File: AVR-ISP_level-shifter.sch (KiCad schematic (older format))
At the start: 24 parts, among them Q1 BSS138, Q2 BSS138, Q3 BSS138, Q4 BSS138, Q5 BSS138, Q6 BSS138, Q7 BSS138, Q8 BSS138, SW1 APEM 25439NH, U1 AMS1117-3.3

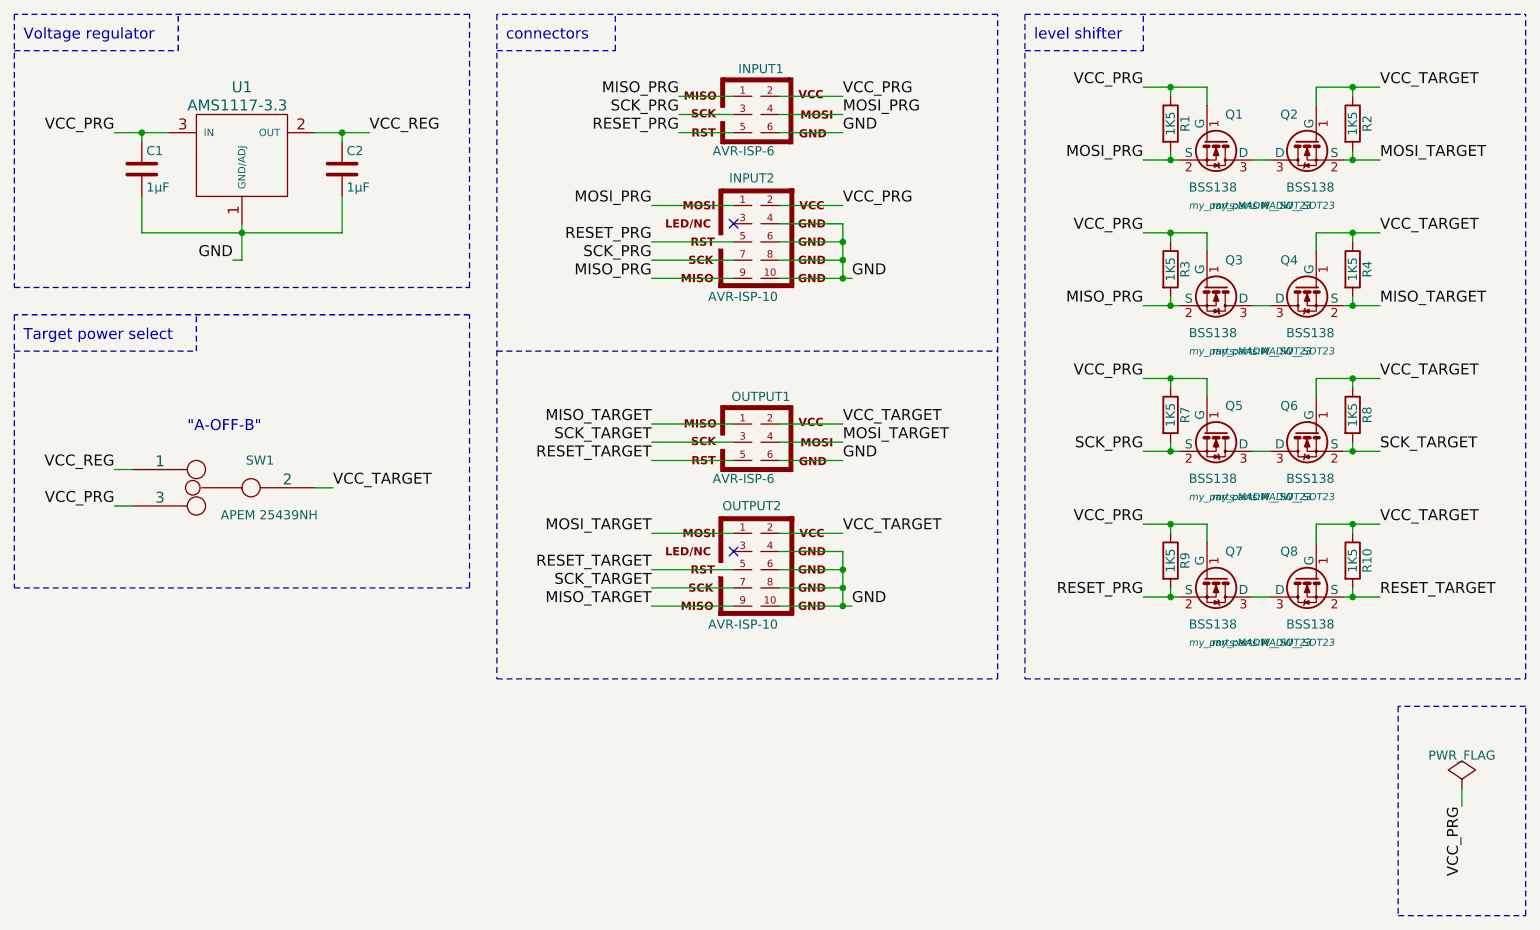
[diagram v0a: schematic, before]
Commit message: Changed a few footprints.
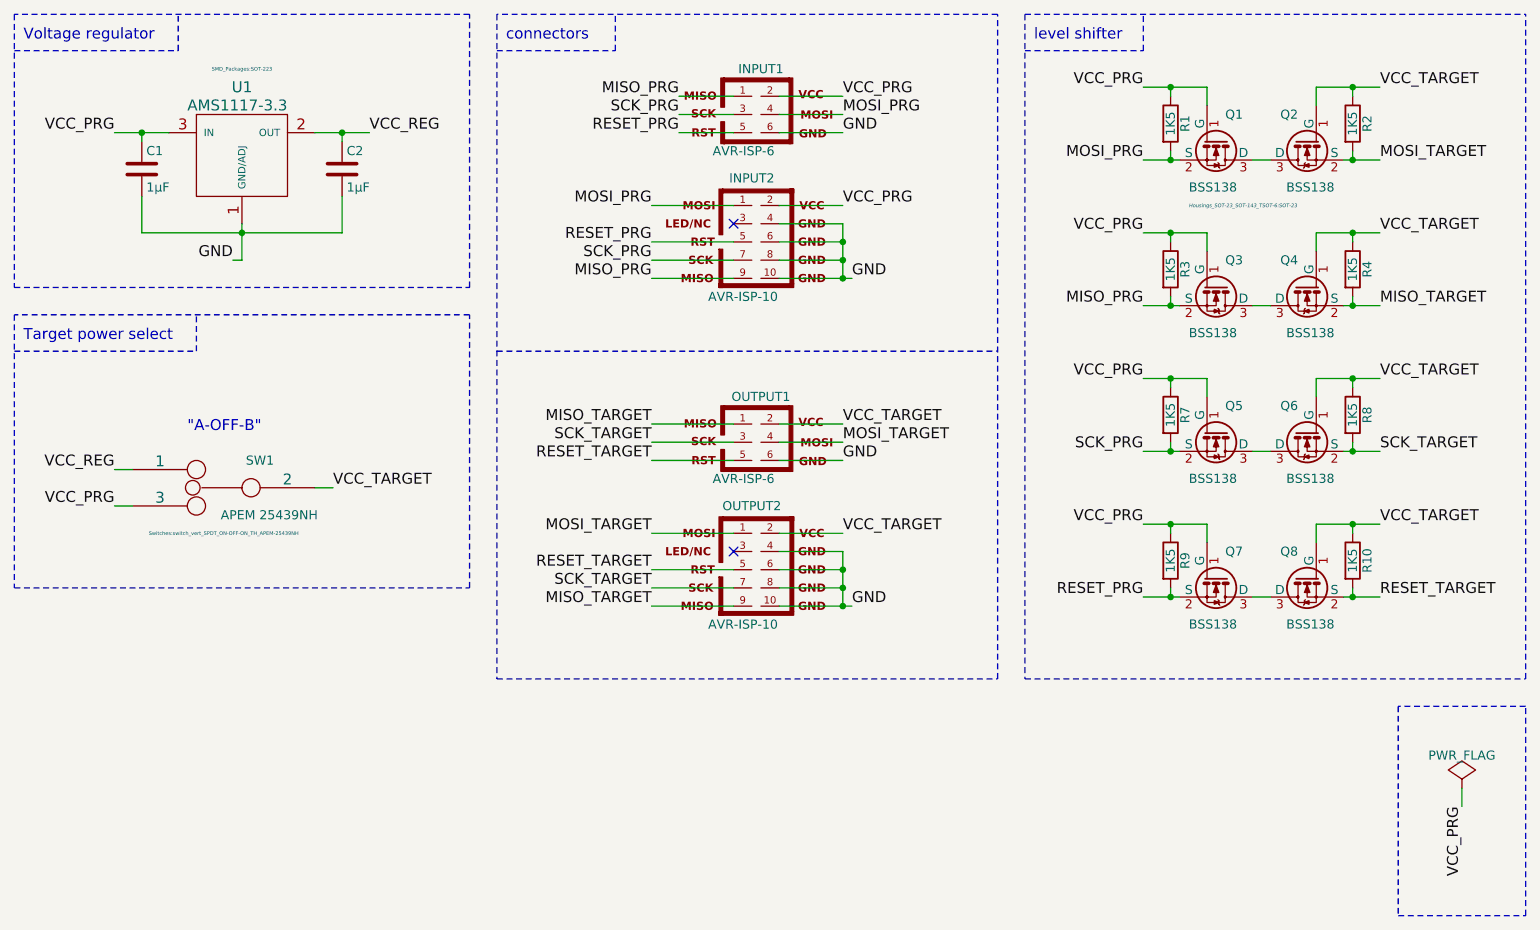
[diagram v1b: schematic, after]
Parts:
- Q1, Q2, Q3, Q4, Q5, Q6, Q7, Q8: footprint my_parts:MADW__SOT23 -> Housings_SOT-23_SOT-143_TSOT-6:SOT-23
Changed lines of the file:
@@
 F 0 "U1" H 3850 2050 60  0000 C CNN
 F 1 "AMS1117-3.3" H 3550 1950 60  0000 L CNN
-F 2 "SMD_Packages:SOT-223" H 3850 1650 60  0001 C CNN
+F 2 "SMD_Packages:SOT-223" H 3850 2150 20  0000 C CNN
 F 3 "" H 3850 1650 60  0000 C CNN
 	1    3850 1650
@@
 F 0 "Q1" V 9050 1600 50  0000 L CNN
 F 1 "BSS138" V 9450 1400 50  0000 L CNN
-F 2 "my_parts:MADW__SOT23" V 9550 1400 39  0000 L CIN
+F 2 "Housings_SOT-23_SOT-143_TSOT-6:SOT-23" V 9550 1400 20  0000 L CIN
 F 3 "" H 9200 1550 50  0000 L CNN
 	1    9200 1550
@@
 F 0 "Q2" V 9550 1600 50  0000 L CNN
 F 1 "BSS138" V 9950 1400 50  0000 L CNN
-F 2 "my_parts:MADW__SOT23" V 10050 1400 39  0000 L CIN
+F 2 "Housings_SOT-23_SOT-143_TSOT-6:SOT-23" V 10050 1400 20  0001 L CIN
 F 3 "" H 9700 1550 50  0000 L CNN
 	1    9700 1550
@@
 F 0 "Q3" V 9050 2400 50  0000 L CNN
 F 1 "BSS138" V 9450 2200 50  0000 L CNN
-F 2 "my_parts:MADW__SOT23" V 9550 2200 39  0000 L CIN
+F 2 "Housings_SOT-23_SOT-143_TSOT-6:SOT-23" V 9550 2200 20  0001 L CIN
 F 3 "" H 9200 2350 50  0000 L CNN
 	1    9200 2350
@@
 F 0 "Q4" V 9550 2400 50  0000 L CNN
 F 1 "BSS138" V 9950 2200 50  0000 L CNN
-F 2 "my_parts:MADW__SOT23" V 10050 2200 39  0000 L CIN
+F 2 "Housings_SOT-23_SOT-143_TSOT-6:SOT-23" V 10050 2200 20  0001 L CIN
 F 3 "" H 9700 2350 50  0000 L CNN
 	1    9700 2350
@@
 F 0 "Q5" V 9050 3200 50  0000 L CNN
 F 1 "BSS138" V 9450 3000 50  0000 L CNN
-F 2 "my_parts:MADW__SOT23" V 9550 3000 39  0000 L CIN
+F 2 "Housings_SOT-23_SOT-143_TSOT-6:SOT-23" V 9550 3000 20  0001 L CIN
 F 3 "" H 9200 3150 50  0000 L CNN
 	1    9200 3150
@@
 F 0 "Q6" V 9550 3200 50  0000 L CNN
 F 1 "BSS138" V 9950 3000 50  0000 L CNN
-F 2 "my_parts:MADW__SOT23" V 10050 3000 39  0000 L CIN
+F 2 "Housings_SOT-23_SOT-143_TSOT-6:SOT-23" V 10050 3000 20  0001 L CIN
 F 3 "" H 9700 3150 50  0000 L CNN
 	1    9700 3150
@@
 F 0 "SW1" H 3551 3600 50  0000 C CNN
 F 1 "APEM 25439NH" H 3500 3300 50  0000 C CNN
-F 2 "Switches:switch_vert_SPDT_ON-OFF-ON_TH_APEM-25439NH" H 3750 3450 60  0001 C CNN
+F 2 "Switches:switch_vert_SPDT_ON-OFF-ON_TH_APEM-25439NH" H 3750 3200 20  0000 C CNN
 F 3 "" H 3750 3450 60  0000 C CNN
 	1    3750 3450
@@
 F 0 "Q7" V 9050 4000 50  0000 L CNN
 F 1 "BSS138" V 9450 3800 50  0000 L CNN
-F 2 "my_parts:MADW__SOT23" V 9550 3800 39  0000 L CIN
+F 2 "Housings_SOT-23_SOT-143_TSOT-6:SOT-23" V 9550 3800 20  0001 L CIN
 F 3 "" H 9200 3950 50  0000 L CNN
 	1    9200 3950
@@
 F 0 "Q8" V 9550 4000 50  0000 L CNN
 F 1 "BSS138" V 9950 3800 50  0000 L CNN
-F 2 "my_parts:MADW__SOT23" V 10050 3800 39  0000 L CIN
+F 2 "Housings_SOT-23_SOT-143_TSOT-6:SOT-23" V 10050 3800 20  0001 L CIN
 F 3 "" H 9700 3950 50  0000 L CNN
 	1    9700 3950
